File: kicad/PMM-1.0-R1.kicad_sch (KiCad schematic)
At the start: 6 parts, among them U11 TPS22917DBV, U2 BQ25895RTW, U4 BQ27441-G1, U6 TPS61089, U9 STM32C031C4T6

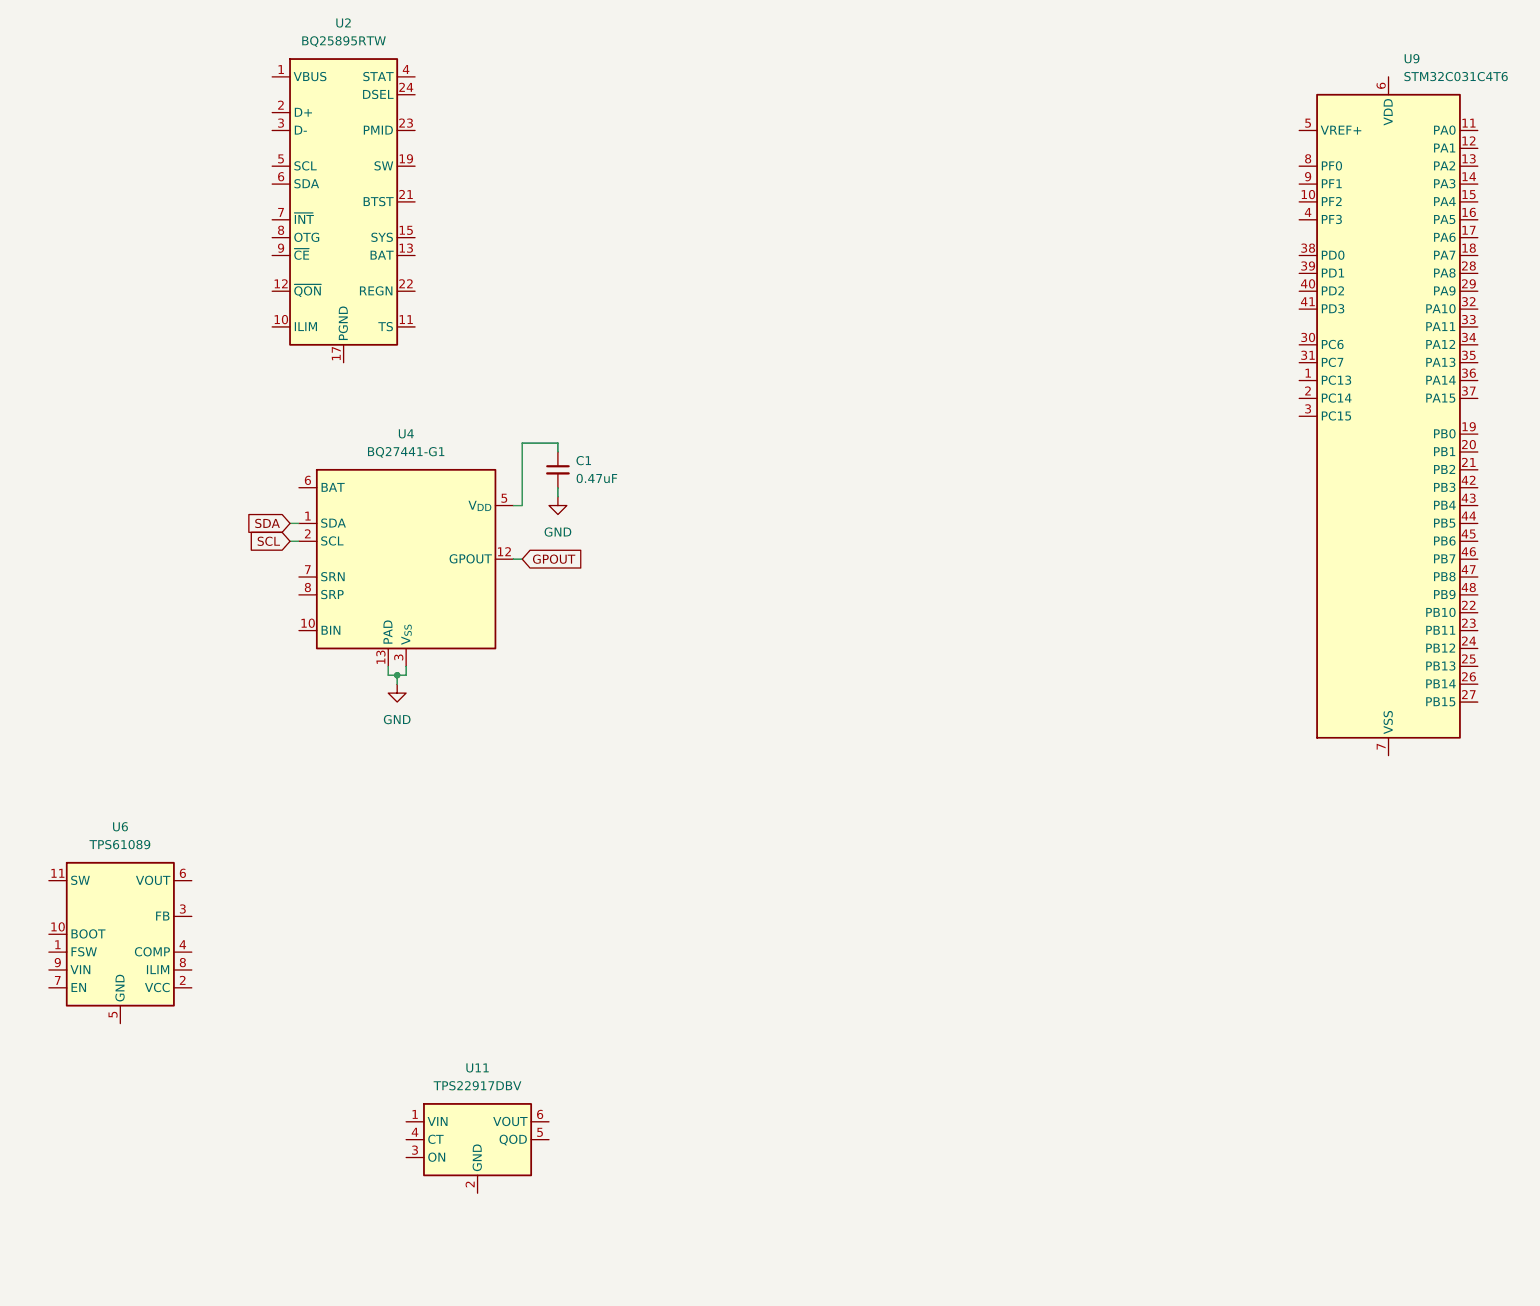
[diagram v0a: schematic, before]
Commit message: add simulations
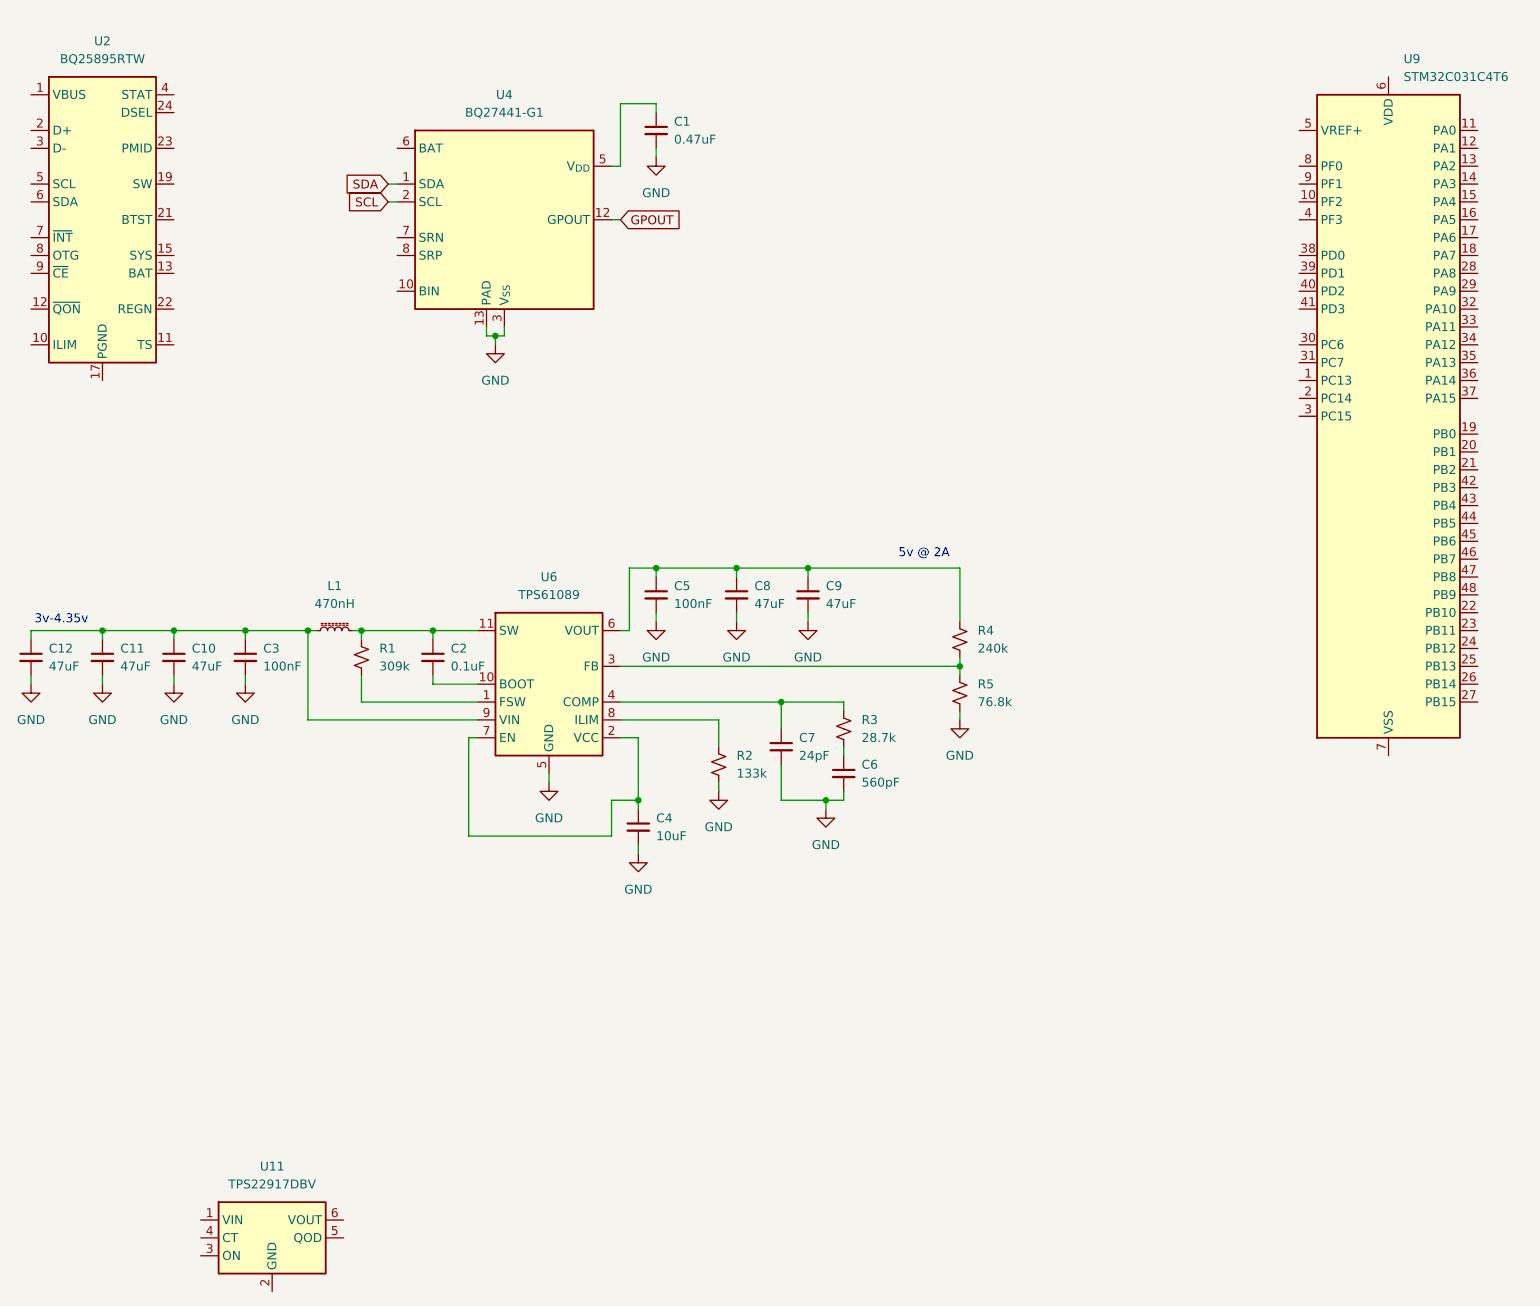
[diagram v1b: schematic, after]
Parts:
- added C10, C11, C12, C8, C9: 47uF, symbol Device:C_Small
- added C2: 0.1uF, symbol Device:C_Small
- added C3, C5: 100nF, symbol Device:C_Small
- added C4: 10uF, symbol Device:C_Small
- added C6: 560pF, symbol Device:C_Small
- added C7: 24pF, symbol Device:C_Small
- added L1: 470nH, symbol Device:L_Ferrite_Small
- added R1: 309k, symbol Device:R_Small_US
- added R2: 133k, symbol Device:R_Small_US
- added R3: 28.7k, symbol Device:R_Small_US
- added R4: 240k, symbol Device:R_Small_US
- added R5: 76.8k, symbol Device:R_Small_US
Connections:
- net GND: now also U6.5 (GND), C10.2, C11.2, C12.2, C3.2, C4.2, C5.2, C6.2, C7.2, C8.2, C9.2, R2.2, R5.2
- net at U6.1 (FSW): now also R1.2
- net at U6.10 (BOOT): now also C2.2
- net at U6.11 (SW): now also C2.1, L1.2, R1.1
- net at U6.2 (VCC): now also U6.7 (EN), C4.1
- net at U6.3 (FB): now also R4.2, R5.1
- net at U6.4 (COMP): now also C7.1, R3.1
- net at U6.6 (VOUT): now also C5.1, C8.1, C9.1, R4.1
- net at U6.8 (ILIM): now also R2.1
- net at U6.9 (VIN): now also C10.1, C11.1, C12.1, C3.1, L1.1
- new net: C6.1, R3.2
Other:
- note added: "3v-4.35v"
- note added: "5v @ 2A"
- moved on the sheet: C1, U11, U2, U4, U6
